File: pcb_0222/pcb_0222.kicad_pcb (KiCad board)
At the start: 2 copper layers, 80 x 70 mm, 95 parts, among them J1 S2P-VH, J2 SM02B-PASS-TBT, J3 SM02B-PASS-TBT, J4 SM08B-PASS-TBT, J5 TC-2030-IDC, J6 SM08B-PASS-TBT, J7 HEADER_MALE_THT_0.1"_4x1, J8 HEADER_MALE_THT_0.1"_2x1, J9 HEADER_MALE_THT_0.1"_4x1, K1 EE2-3NUH, Q1 BSP170PH6327XTSA1, Q2 BC817-16, U1 LMR54406DBVR, U2 STM32C011F6P6

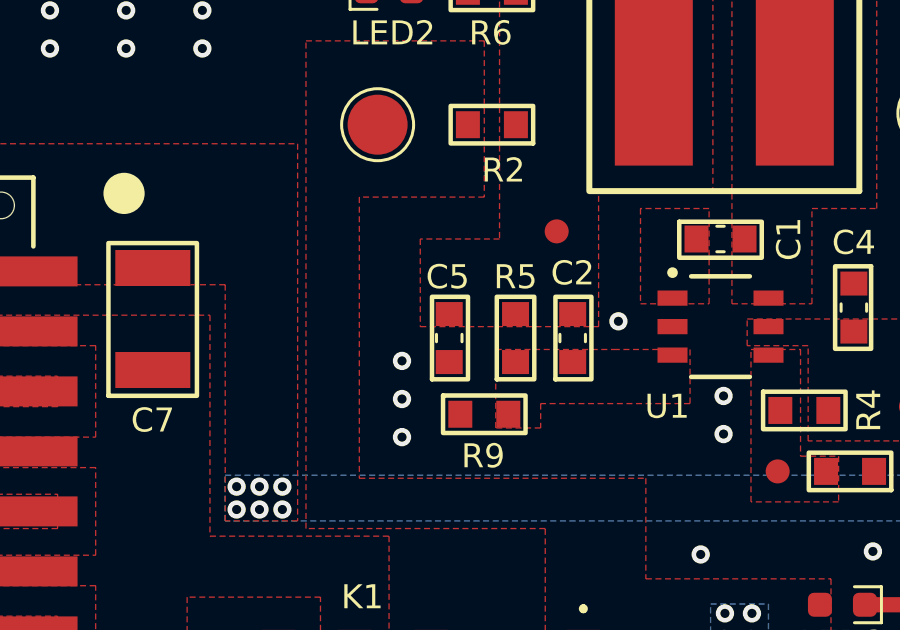
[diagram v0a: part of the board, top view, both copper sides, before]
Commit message: Layout Review Pass
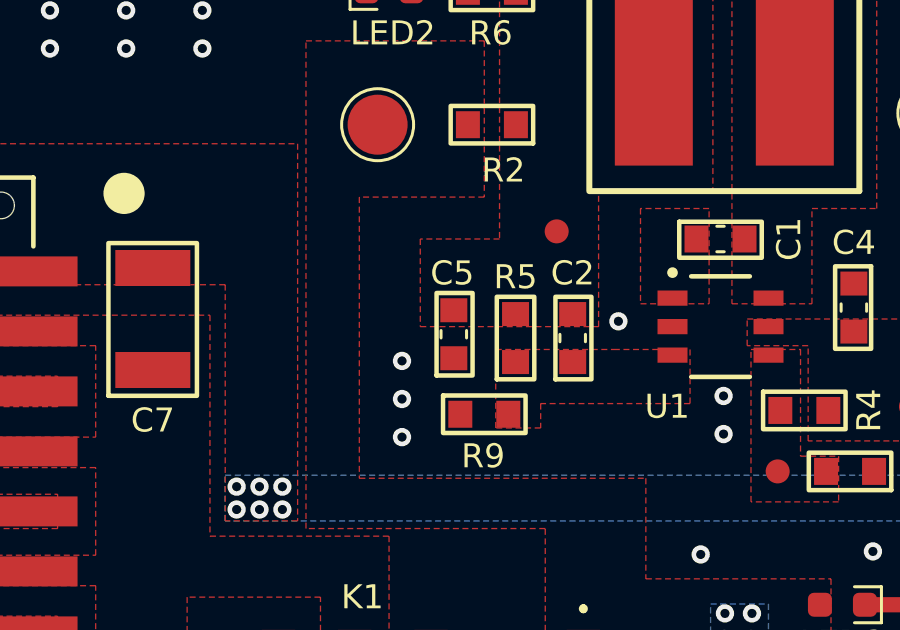
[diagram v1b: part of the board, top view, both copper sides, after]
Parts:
- moved C5 0.20 mm to (140.2, 85.2)
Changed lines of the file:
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@@
 	(title_block
 		(title "UV Floor Sanitization Unit")
-		(date "2026-08-16")
+		(date "2026-08-27")
+		(rev "20260827")
 		(company "Designed by Logic Reliance for Satview Broadband Ltd")
 	)
@@
 		(grid_origin 113.995 137.894)
 		(pcbplotparams
-			(layerselection 0x00000000_00000000_5555555d_55555550)
-			(plot_on_all_layers_selection 0x00000000_00000000_00000008_02000000)
+			(layerselection 0x00000000_00000000_5555555f_5755f5ff)
+			(plot_on_all_layers_selection 0x00000000_00000000_00000000_00000000)
 			(disableapertmacros no)
 			(usegerberextensions no)
@@
 			(mode 1)
 			(useauxorigin no)
-			(pdf_front_fp_property_popups no)
-			(pdf_back_fp_property_popups no)
-			(pdf_metadata no)
+			(pdf_front_fp_property_popups yes)
+			(pdf_back_fp_property_popups yes)
+			(pdf_metadata yes)
 			(pdf_single_document no)
 			(dxfpolygonmode yes)
@@
 			(crossoutdnponfab no)
 			(subtractmaskfromsilk no)
-			(outputformat 4)
+			(outputformat 1)
 			(mirror no)
-			(drillshape 2)
+			(drillshape 0)
 			(scaleselection 1)
-			(outputdirectory "outputs/Manufacture/20260816-P_0222_manufacture/DWG/")
+			(outputdirectory "outputs/Manufacture/20260827-P_0222_manufacture/DRILLS/")
 		)
 	)
@@
 	(footprint "passives_smd:C_0603"
 		(layer "F.Cu")
-		(at 140.0046 85.316 90)
+		(at 140.157 85.189 90)
 		(descr "<b>CAPACITOR</b>")
 		(property "Reference" "C5"
@@
 	)
 	(zone
-		(net "Net-(J9-Pad3)")
-		(layer "F.Cu")
-		(hatch none 0.1)
-		(priority 30000)
-		(attr
-			(teardrop
-				(type padvia)
-			)
-		)
-		(connect_pads yes
-			(clearance 0)
-		)
-		(min_thickness 0.0254)
-		(fill yes
-			(island_removal_mode 1)
-		)
-		(polygon
-			(pts
-				(xy 169.515153 125.0035) (xy 169.515153 125.3845) (xy 170.48442 125.954657) (xy 170.896153 125.194)
-				(xy 170.48442 124.433343)
-			)
-		)
-	)
-	(zone
 		(net "VB_IP")
 		(layer "F.Cu")
@@
 	)
 	(zone
-		(net "/NRST")
-		(layer "F.Cu")
-		(hatch none 0.1)
-		(priority 30004)
-		(attr
-			(teardrop
-				(type padvia)
-			)
-		)
-		(connect_pads yes
-			(clearance 0)
-		)
-		(min_thickness 0.0254)
-		(fill yes
-			(island_removal_mode 1)
-		)
-		(polygon
-			(pts
-				(xy 143.990166 127.2895) (xy 143.990166 126.9085) (xy 143.923904 126.964296) (xy 143.466543 126.224331)
-				(xy 143.151111 126.460911) (xy 142.914531 126.776343) (xy 143.654496 127.233704) (xy 143.7892 127.2895)
-			)
-		)
-	)
-	(zone
 		(net "+3V3")
 		(layer "F.Cu")
@@
 	)
 	(zone
+		(net "Net-(J7-Pad2)")
+		(layer "F.Cu")
+		(hatch none 0.1)
+		(priority 30002)
+		(attr
+			(teardrop
+				(type padvia)
+			)
+		)
+		(connect_pads yes
+			(clearance 0)
+		)
+		(min_thickness 0.0254)
+		(fill yes
+			(island_removal_mode 1)
+		)
+		(polygon
+			(pts
+				(xy 169.515153 115.1991) (xy 169.515153 115.5801) (xy 170.48442 116.175657) (xy 170.896153 115.3896)
+				(xy 170.48442 114.654343)
+			)
+		)
+	)
+	(zone
 		(net "VB_IP")
 		(layer "F.Cu")
@@
 	)
 	(zone
+		(net "Net-(J7-Pad3)")
+		(layer "F.Cu")
+		(hatch none 0.1)
+		(priority 30003)
+		(attr
+			(teardrop
+				(type padvia)
+			)
+		)
+		(connect_pads yes
+			(clearance 0)
+		)
+		(min_thickness 0.0254)
+		(fill yes
+			(island_removal_mode 1)
+		)
+		(polygon
+			(pts
+				(xy 169.515153 112.6845) (xy 169.515153 113.0655) (xy 170.48442 113.635657) (xy 170.896153 112.875)
+				(xy 170.48442 112.114343)
+			)
+		)
+	)
+	(zone
 		(net "GND")
 		(layer "F.Cu")
@@
 	)
 	(zone
-		(net "Net-(J5-SWCLK)")
-		(layer "F.Cu")
-		(hatch none 0.1)
-		(priority 30005)
-		(attr
-			(teardrop
-				(type padvia)
-			)
-		)
-		(connect_pads yes
-			(clearance 0)
-		)
-		(min_thickness 0.0254)
-		(fill yes
-			(island_removal_mode 1)
-		)
-		(polygon
-			(pts
-				(xy 141.195103 128.15369) (xy 141.46451 128.423097) (xy 142.034862 128.097731) (xy 141.887289 127.730911)
-				(xy 141.520469 127.583338)
-			)
-		)
-	)
-	(zone
 		(net "+3V3")
 		(layer "F.Cu")
@@
 	)
 	(zone
-		(net "Net-(J5-SWDIO)")
+		(net "Net-(J9-Pad2)")
 		(layer "F.Cu")
 		(hatch none 0.1)
-		(priority 30006)
+		(priority 30001)
 		(attr
 			(teardrop
@@
 		(polygon
 			(pts
-				(xy 140.079968 126.0195) (xy 140.079968 126.4005) (xy 140.223868 126.48559) (xy 140.710888 126.21)
-				(xy 140.665588 126.073668)
+				(xy 169.515153 127.5435) (xy 169.515153 127.9245) (xy 170.48442 128.494657) (xy 170.896153 127.734)
+				(xy 170.48442 126.973343)
 			)
 		)
@@
 	)
 	(zone
+		(net "Net-(J5-SWCLK)")
+		(layer "F.Cu")
+		(hatch none 0.1)
+		(priority 30005)
+		(attr
+			(teardrop
+				(type padvia)
+			)
+		)
+		(connect_pads yes
+			(clearance 0)
+		)
+		(min_thickness 0.0254)
+		(fill yes
+			(island_removal_mode 1)
+		)
+		(polygon
+			(pts
+				(xy 141.195103 128.15369) (xy 141.46451 128.423097) (xy 142.034862 128.097731) (xy 141.887289 127.730911)
+				(xy 141.520469 127.583338)
+			)
+		)
+	)
+	(zone
 		(net "+3V3")
 		(layer "F.Cu")
@@
 	)
 	(zone
+		(net "Net-(J9-Pad3)")
+		(layer "F.Cu")
+		(hatch none 0.1)
+		(priority 30000)
+		(attr
+			(teardrop
+				(type padvia)
+			)
+		)
+		(connect_pads yes
+			(clearance 0)
+		)
+		(min_thickness 0.0254)
+		(fill yes
+			(island_removal_mode 1)
+		)
+		(polygon
+			(pts
+				(xy 169.515153 125.0035) (xy 169.515153 125.3845) (xy 170.48442 125.954657) (xy 170.896153 125.194)
+				(xy 170.48442 124.433343)
+			)
+		)
+	)
+	(zone
 		(net "Net-(U1-CB)")
 		(layer "F.Cu")
@@
 	)
 	(zone
-		(net "Net-(J9-Pad2)")
-		(layer "F.Cu")
-		(hatch none 0.1)
-		(priority 30001)
-		(attr
-			(teardrop
-				(type padvia)
-			)
-		)
-		(connect_pads yes
-			(clearance 0)
-		)
-		(min_thickness 0.0254)
-		(fill yes
-			(island_removal_mode 1)
-		)
-		(polygon
-			(pts
-				(xy 169.515153 127.5435) (xy 169.515153 127.9245) (xy 170.48442 128.494657) (xy 170.896153 127.734)
-				(xy 170.48442 126.973343)
-			)
-		)
-	)
-	(zone
 		(net "Net-(U1-EN)")
 		(layer "F.Cu")
@@
 	)
 	(zone
-		(net "Net-(J7-Pad2)")
+		(net "Net-(J5-SWDIO)")
 		(layer "F.Cu")
 		(hatch none 0.1)
-		(priority 30002)
+		(priority 30006)
 		(attr
 			(teardrop
@@
 		(polygon
 			(pts
-				(xy 169.515153 115.1991) (xy 169.515153 115.5801) (xy 170.48442 116.175657) (xy 170.896153 115.3896)
-				(xy 170.48442 114.654343)
+				(xy 140.079968 126.0195) (xy 140.079968 126.4005) (xy 140.223868 126.48559) (xy 140.710888 126.21)
+				(xy 140.665588 126.073668)
 			)
 		)
 	)
 	(zone
-		(net "Net-(J7-Pad3)")
+		(net "/NRST")
 		(layer "F.Cu")
 		(hatch none 0.1)
-		(priority 30003)
+		(priority 30004)
 		(attr
 			(teardrop
@@
 		(polygon
 			(pts
-				(xy 169.515153 112.6845) (xy 169.515153 113.0655) (xy 170.48442 113.635657) (xy 170.896153 112.875)
-				(xy 170.48442 112.114343)
+				(xy 143.990166 127.2895) (xy 143.990166 126.9085) (xy 143.923904 126.964296) (xy 143.466543 126.224331)
+				(xy 143.151111 126.460911) (xy 142.914531 126.776343) (xy 143.654496 127.233704) (xy 143.7892 127.2895)
 			)
 		)
@@
 	)
 	(zone
-		(net "/SWCLK")
-		(layer "B.Cu")
-		(hatch none 0.1)
-		(priority 30000)
-		(attr
-			(teardrop
-				(type padvia)
-			)
-		)
-		(connect_pads yes
-			(clearance 0)
-		)
-		(min_thickness 0.0254)
-		(fill yes
-			(island_removal_mode 1)
-		)
-		(polygon
-			(pts
-				(xy 148.9327 130.481973) (xy 148.5517 130.481973) (xy 148.065415 131.409098) (xy 148.7422 131.802973)
-				(xy 149.520585 131.409098)
-			)
-		)
-	)
-	(zone
 		(net "VB")
 		(layer "B.Cu")
@@
 			)
 		)
+	)
+	(zone
+		(net "/SWCLK")
+		(layer "B.Cu")
+		(hatch none 0.1)
+		(priority 30000)
+		(attr
+			(teardrop
+				(type padvia)
+			)
+		)
+		(connect_pads yes
+			(clearance 0)
+		)
+		(min_thickness 0.0254)
+		(fill yes
+			(island_removal_mode 1)
+		)
+		(polygon
+			(pts
+				(xy 148.9327 130.481973) (xy 148.5517 130.481973) (xy 148.065415 131.409098) (xy 148.7422 131.802973)
+				(xy 149.520585 131.409098)
+			)
+		)
